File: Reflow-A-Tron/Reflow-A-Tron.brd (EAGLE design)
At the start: 97.8 x 62.2 mm, 40 parts, among them IC1 ATMEGA644-10PU, J2 HOT, J3 NEUTRAL, Q1 FOXSLF/200-20, Q2 BSS123, U1 FT230X, U2 L4941BDT-TRDPAK-3, U4 MAX6675

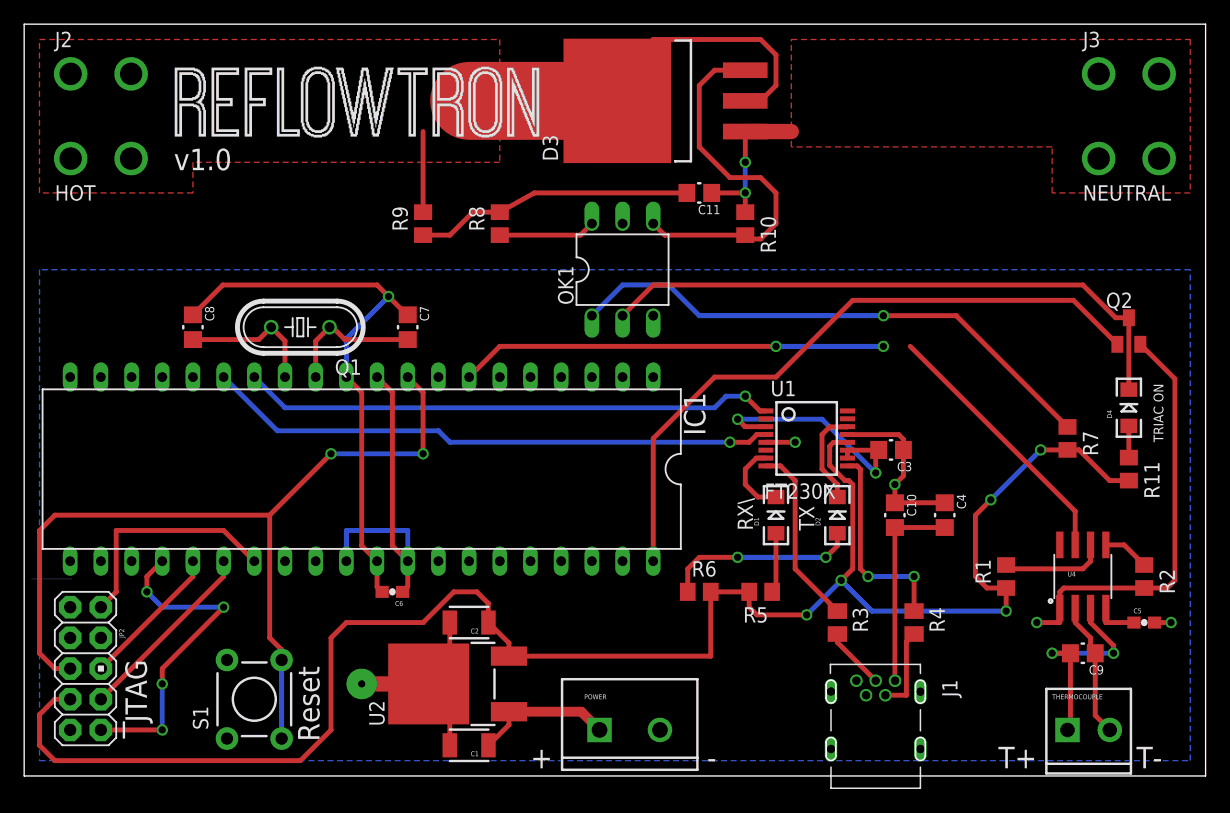
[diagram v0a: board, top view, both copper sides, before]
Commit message: Fix shit
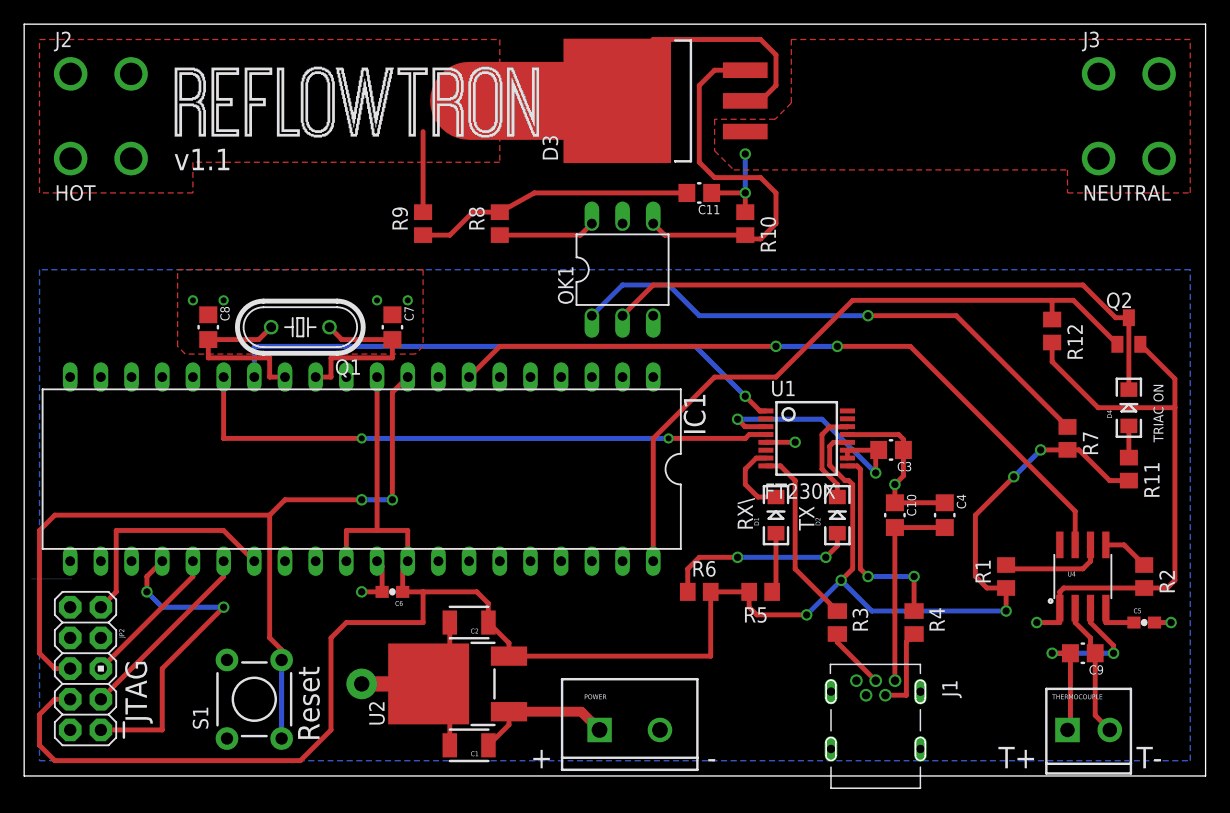
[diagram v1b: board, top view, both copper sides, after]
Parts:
- added R12: 10k, resistor:R0805
- moved C7 1.27 mm to (30.5, 37.1)
- moved C8 1.27 mm to (15.2, 37.1)
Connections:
- removed net GND-MCU: C6.2, C7.1, C8.1, IC1.11, IC1.31
- removed net VCC-MCU: C6.1, IC1.10, IC1.30, IC1.32
- net 5V: now also C6.1, IC1.10, IC1.30, IC1.32
- net GND: now also C6.2, C7.1, C8.1, IC1.11, IC1.31, R12.2
- net TRIAC-CTRL: now also R12.1
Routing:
- net GND-MCU: track 46.9 -> 0.00 mm, vias 1 -> 0
- net VCC-MCU: track 29.2 -> 0.00 mm
- net 5V: track 149.7 -> 178.4 mm
- net GND: track 73.4 -> 91.1 mm, vias 5 -> 10
- net NEUTRAL: track 13.6 -> 7.92 mm
- net XTAL1: track 11.5 -> 15.1 mm
- net XTAL2: track 11.6 -> 15.1 mm
- net N$9: track 44.3 -> 47.1 mm
- net N$10: track 47.4 -> 50.1 mm, vias 1 -> 2
- net MISO: track 57.4 -> 59.7 mm
- net TRIAC-CTRL: track 54.8 -> 56.4 mm
- net N$14: track 31.0 -> 31.7 mm
- net TCK: vias 4 -> 2
- added copper zone on layer 1, net GND
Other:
- board text added: "v1.1"
- board text removed: "v1.0"

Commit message: More fixes
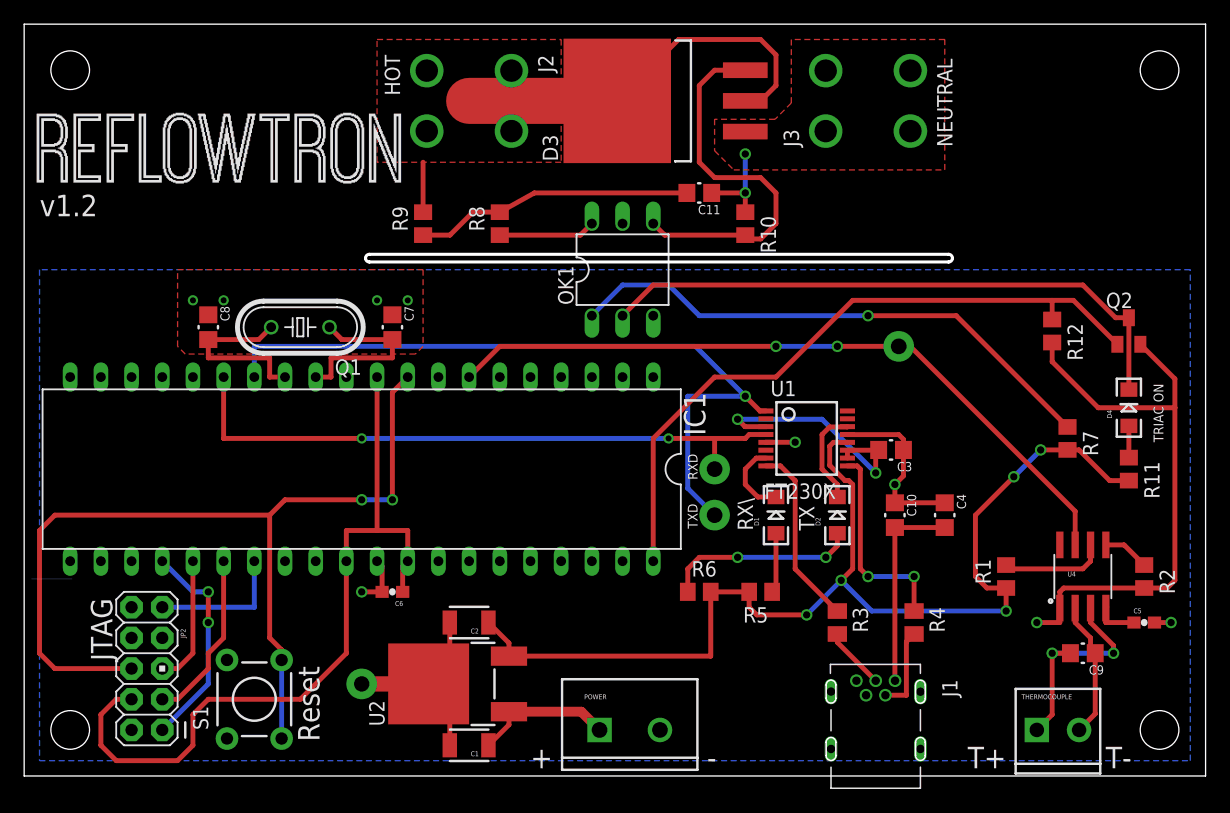
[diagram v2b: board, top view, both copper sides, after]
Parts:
- moved J2 30.5 mm to (36.8, 55.9), turned to 270 degrees
- moved J3 21.6 mm to (69.8, 55.9), turned to 90 degrees
- moved JP2 5.08 mm to (10.2, 8.89)
- moved THERMOCOUPLE 2.54 mm to (83.8, 3.81)
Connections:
- net N$10 renamed RXD
- net N$9 renamed TXD
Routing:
- net 5V: track 178.4 -> 159.0 mm
- net TXD: track 47.1 -> 62.6 mm, vias 1 -> 2
- net TCK: track 27.3 -> 17.9 mm
- net TDI: track 19.4 -> 11.4 mm
- net RESET: track 73.1 -> 78.2 mm
- net HOT: track 41.5 -> 37.8 mm
- net RXD: track 50.1 -> 52.6 mm, vias 2 -> 3
- net TMS: track 12.0 -> 10.7 mm
- net TDO: track 15.6 -> 14.3 mm
- net MISO: vias 2 -> 3
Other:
- outline, holes or cut-outs redrawn
- board text added: "RXD"
- board text added: "TXD"
- board text added: "v1.2"
- board text removed: "v1.1"

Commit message: Add custom lib, still needs more work.
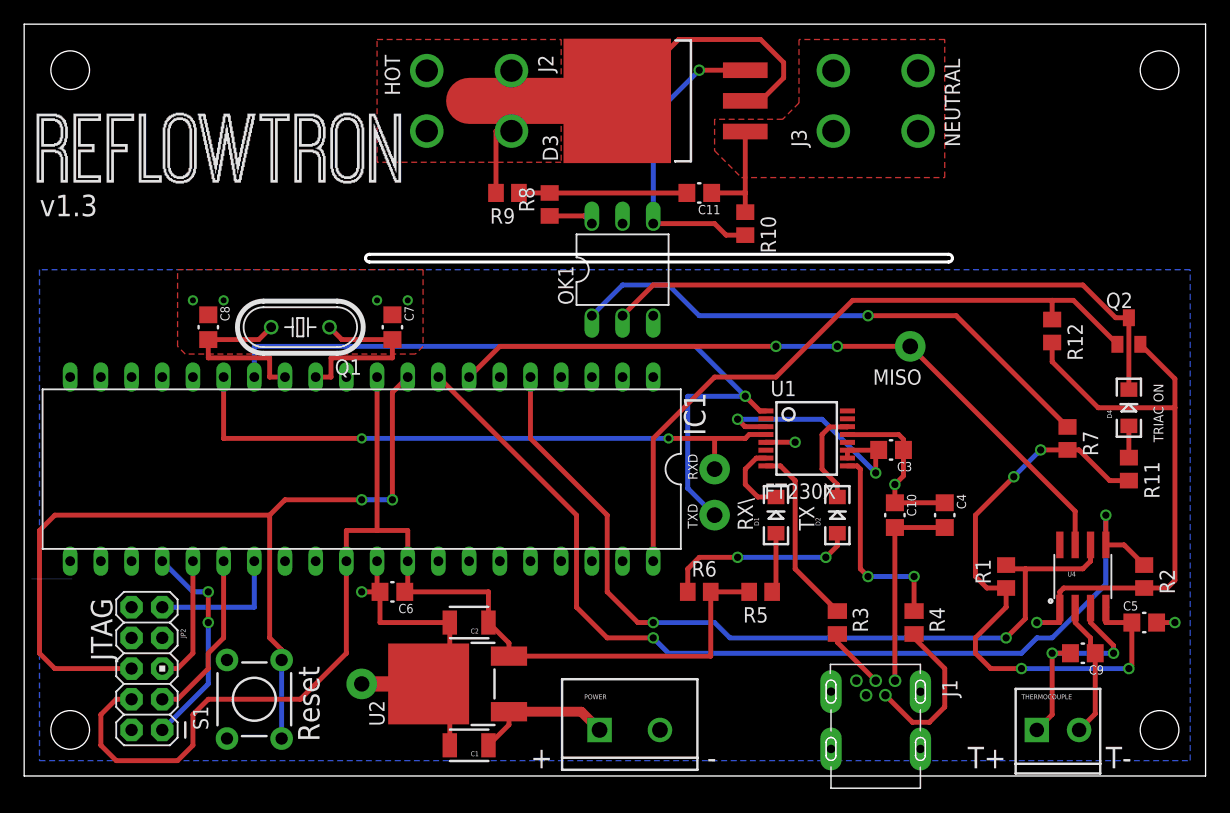
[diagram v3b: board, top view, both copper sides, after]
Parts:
- C5, C6: value 0.1uF -> 10nF; device SparkFun-Capacitors:0603-CAP -> custom:0805
- J1: device neilbetham:XM7D-0512 -> custom:XM7D-0512
- U1: device neilbetham:SSOP-16 -> custom:SSOP-16
- moved R9 7.43 mm to (40.0, 48.3), turned to 180 degrees
- moved R8 4.42 mm to (43.5, 47.3)
- moved J3 0.64 mm to (70.5, 55.9)
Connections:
- removed net ID: J1.4
- removed net MAX-SCK: IC1.8
- removed net MOSI: IC1.6
- removed net N$1: C5.1, U4.4
- removed net N$2: IC1.5
- net 5V: now also C5.1, U4.4
- net CS: now also IC1.5
- net SCK: now also IC1.8
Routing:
- net SCK: track 3.87 -> 83.6 mm, vias 0 -> 2
- net CS: track 8.72 -> 70.1 mm, vias 0 -> 2
- net N$15: track 23.0 -> 13.9 mm
- net GND: track 91.1 -> 99.5 mm
- net N$3: track 7.07 -> 13.5 mm
- net N$14: track 31.7 -> 26.1 mm, vias 0 -> 1
- net 5V: track 159.0 -> 154.5 mm, vias 5 -> 4
- net N$12: track 8.01 -> 3.76 mm
- net N$1: track 3.63 -> 0.00 mm
- net HOT: track 37.8 -> 40.6 mm
- net NEUTRAL: track 7.92 -> 9.45 mm, vias 2 -> 0
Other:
- board text added: "MISO"
- board text added: "v1.3"
- board text removed: "v1.2"

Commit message: Next rev with more bug fixes
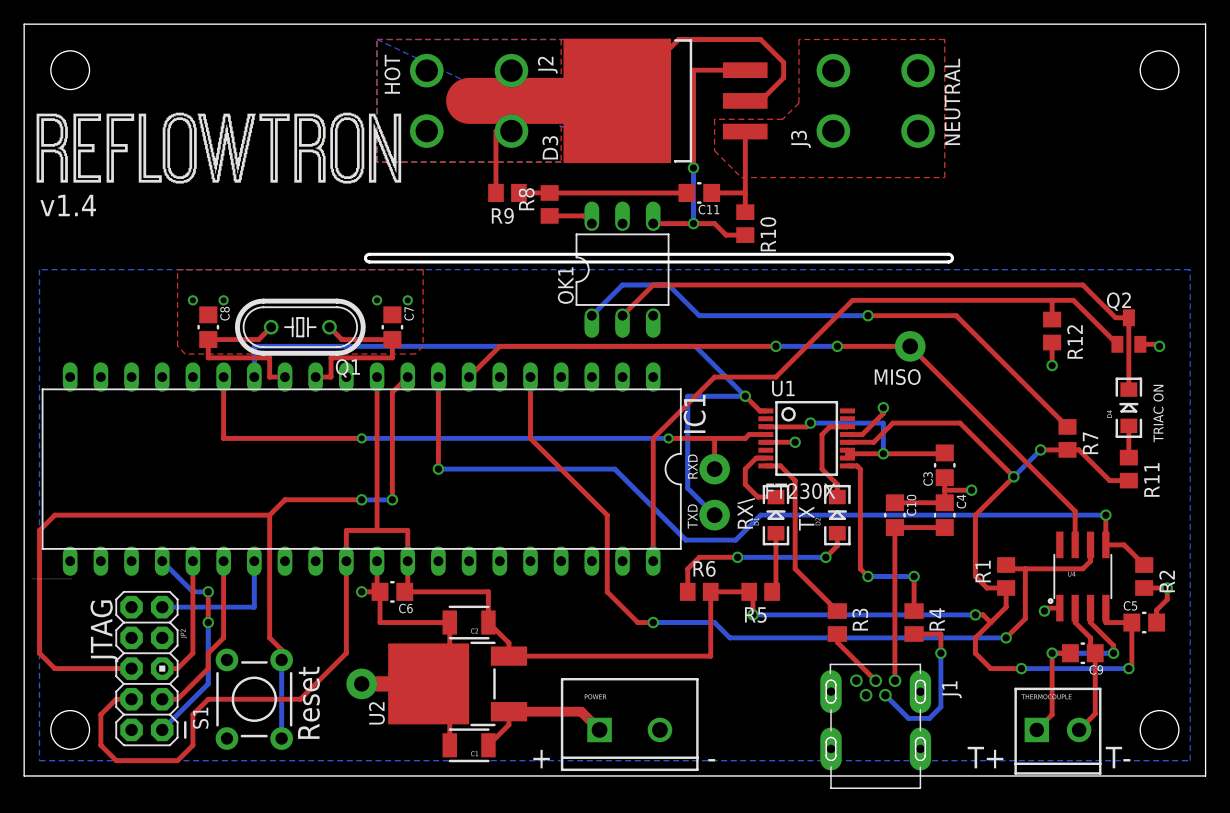
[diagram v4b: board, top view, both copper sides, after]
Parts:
- moved C3 4.62 mm to (76.2, 25.7), turned to 90 degrees
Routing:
- net GND: track 99.5 -> 57.8 mm, vias 10 -> 13
- net 5V: track 154.5 -> 193.0 mm, vias 4 -> 6
- net SCK: track 83.6 -> 72.5 mm
- net N$14: track 26.1 -> 25.0 mm, vias 1 -> 2
- net N$3: track 13.5 -> 14.0 mm, vias 0 -> 1
- added copper zone on layer 16, net HOT
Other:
- board text added: "v1.4"
- board text removed: "v1.3"
